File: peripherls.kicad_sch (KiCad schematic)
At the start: 14 parts, among them SW1 SW_MEC_5E, SW3 SW_MEC_5E, U2 STM32G070KBTx

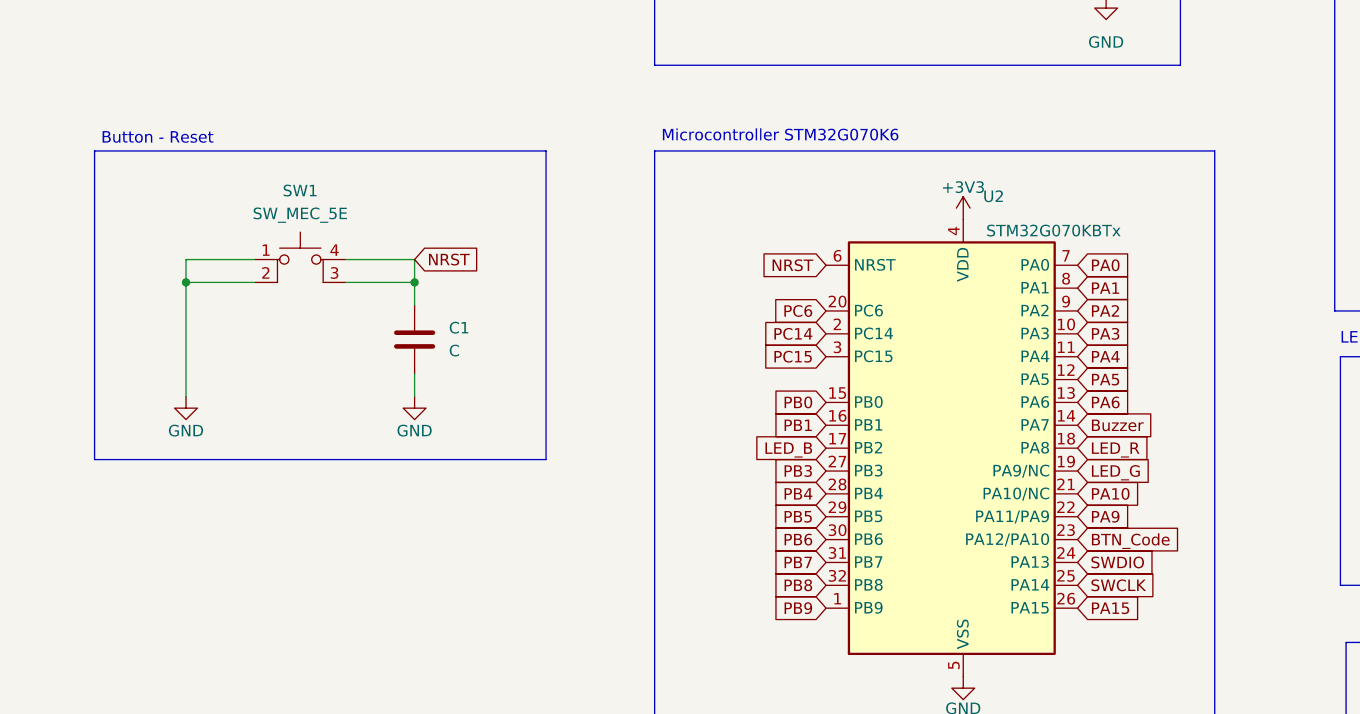
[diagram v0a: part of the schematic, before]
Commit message: [feat] PCB routing
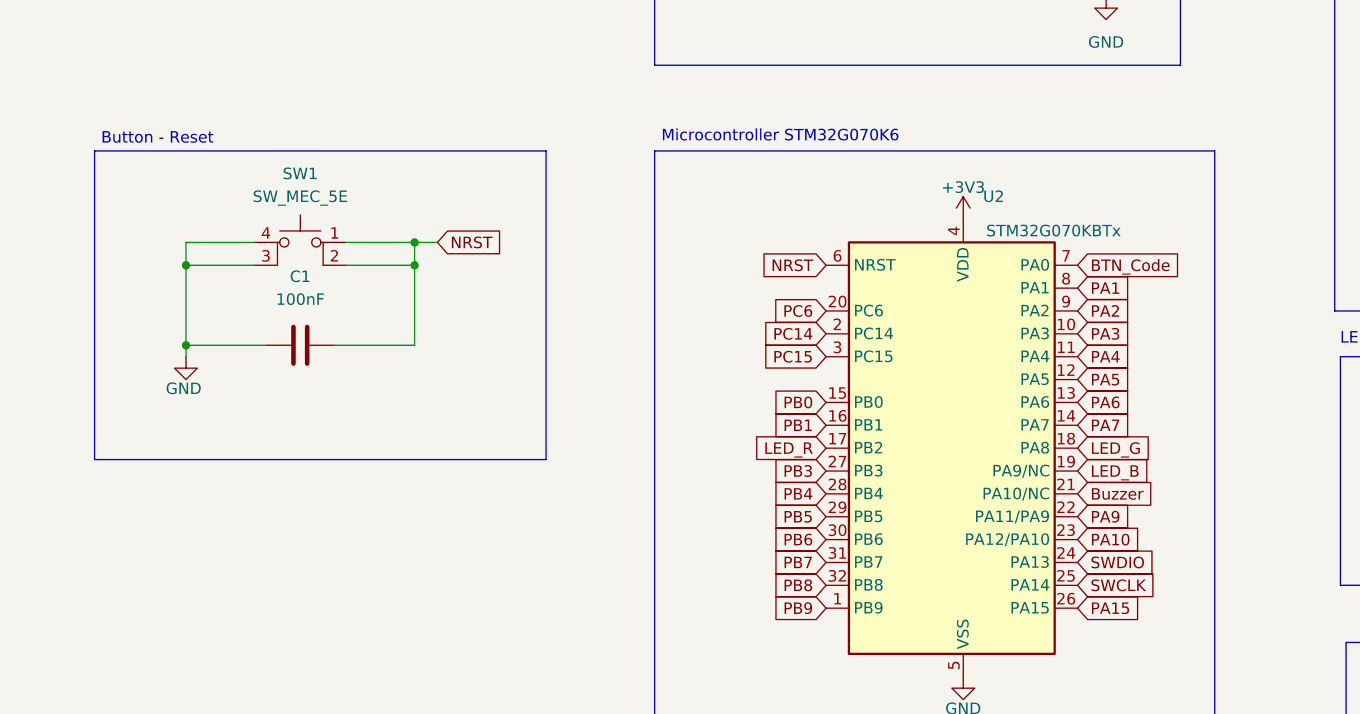
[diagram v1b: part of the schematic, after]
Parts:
- C1: value C -> 100nF
- D1: footprint LED_THT:LED_D1.8mm_W1.8mm_H2.4mm_Horizontal_O3.81mm_Z4.9mm -> LED_THT:LED_D2.0mm_W4.8mm_H2.5mm_FlatTop
- R2: footprint R_Axial_DIN0204_L3.6mm_D1.6mm_P7.62mm_Horizontal -> Resistor_THT:R_Axial_DIN0207_L6.3mm_D2.5mm_P7.62mm_Horizontal
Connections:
- net PA0 is gone; now on net BTN_Code: U2.7 (PA0)
- net BTN_Code: no longer U2.23 (PA12/PA10)
- net Buzzer: now also U2.21 (PA10/NC); no longer U2.14 (PA7)
- net GND: now also C1.1, SW1.3 (K), SW1.4 (A); no longer C1.2, SW1.1, SW1.2
- net LED_B: now also U2.19 (PA9/NC); no longer U2.17 (PB2)
- net LED_G: now also U2.18 (PA8); no longer U2.19 (PA9/NC)
- net LED_R: now also U2.17 (PB2); no longer U2.18 (PA8)
- net NRST: now also C1.2, SW1.1, SW1.2; no longer C1.1, SW1.3 (K), SW1.4 (A)
- net PA10: now also U2.23 (PA12/PA10); no longer U2.21 (PA10/NC)
- new net PA7: U2.14 (PA7)
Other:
- moved on the sheet: C1, SW1

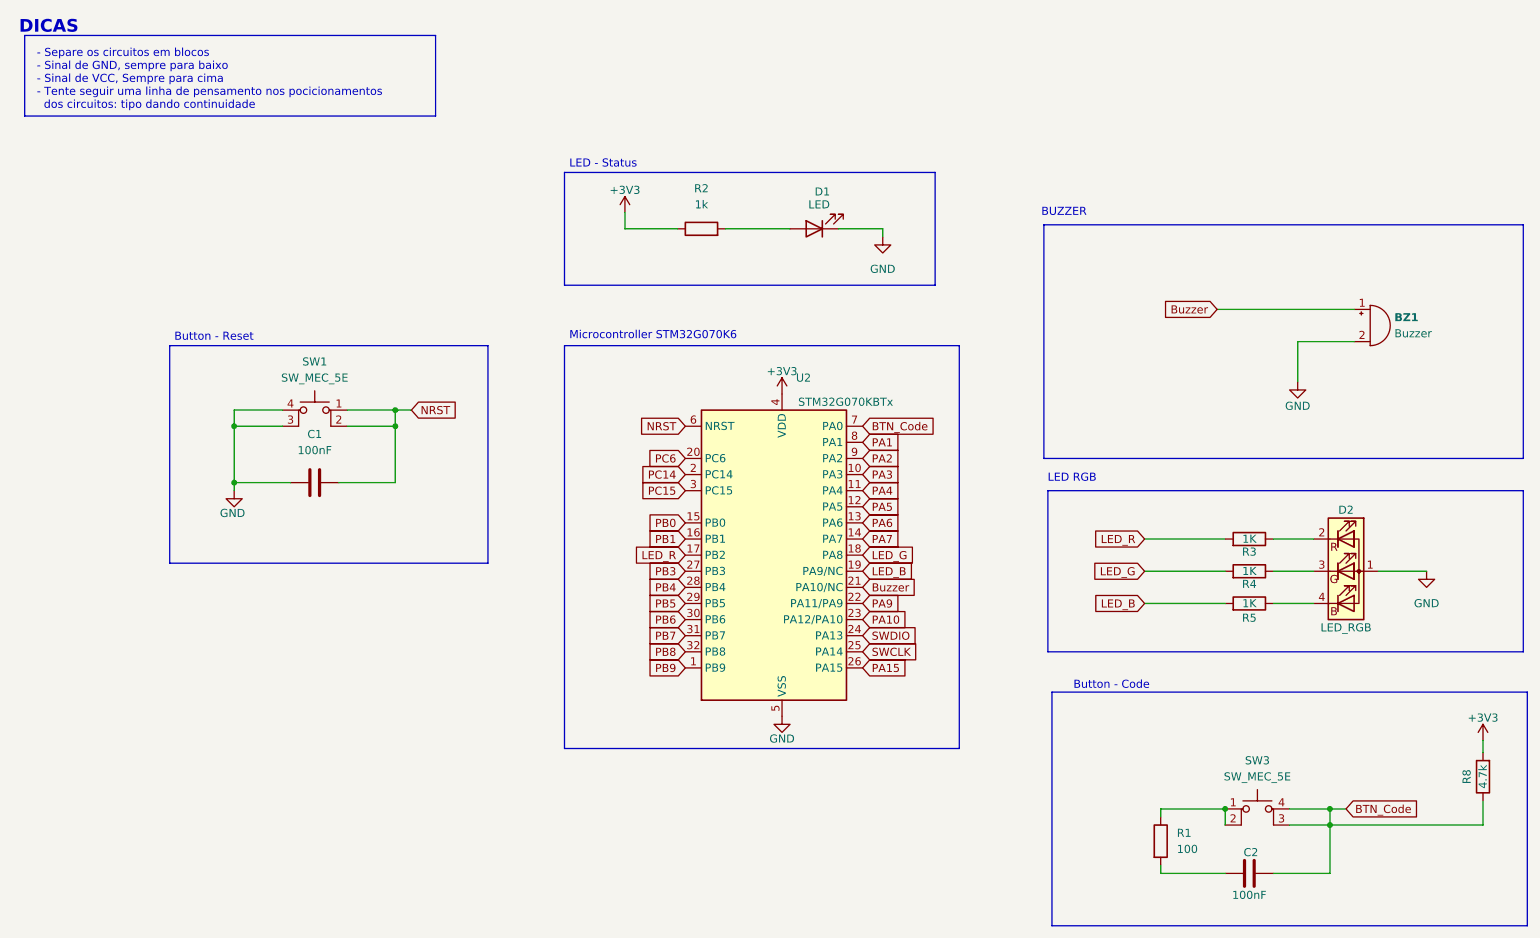
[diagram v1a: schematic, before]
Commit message: Modifying footprint positions
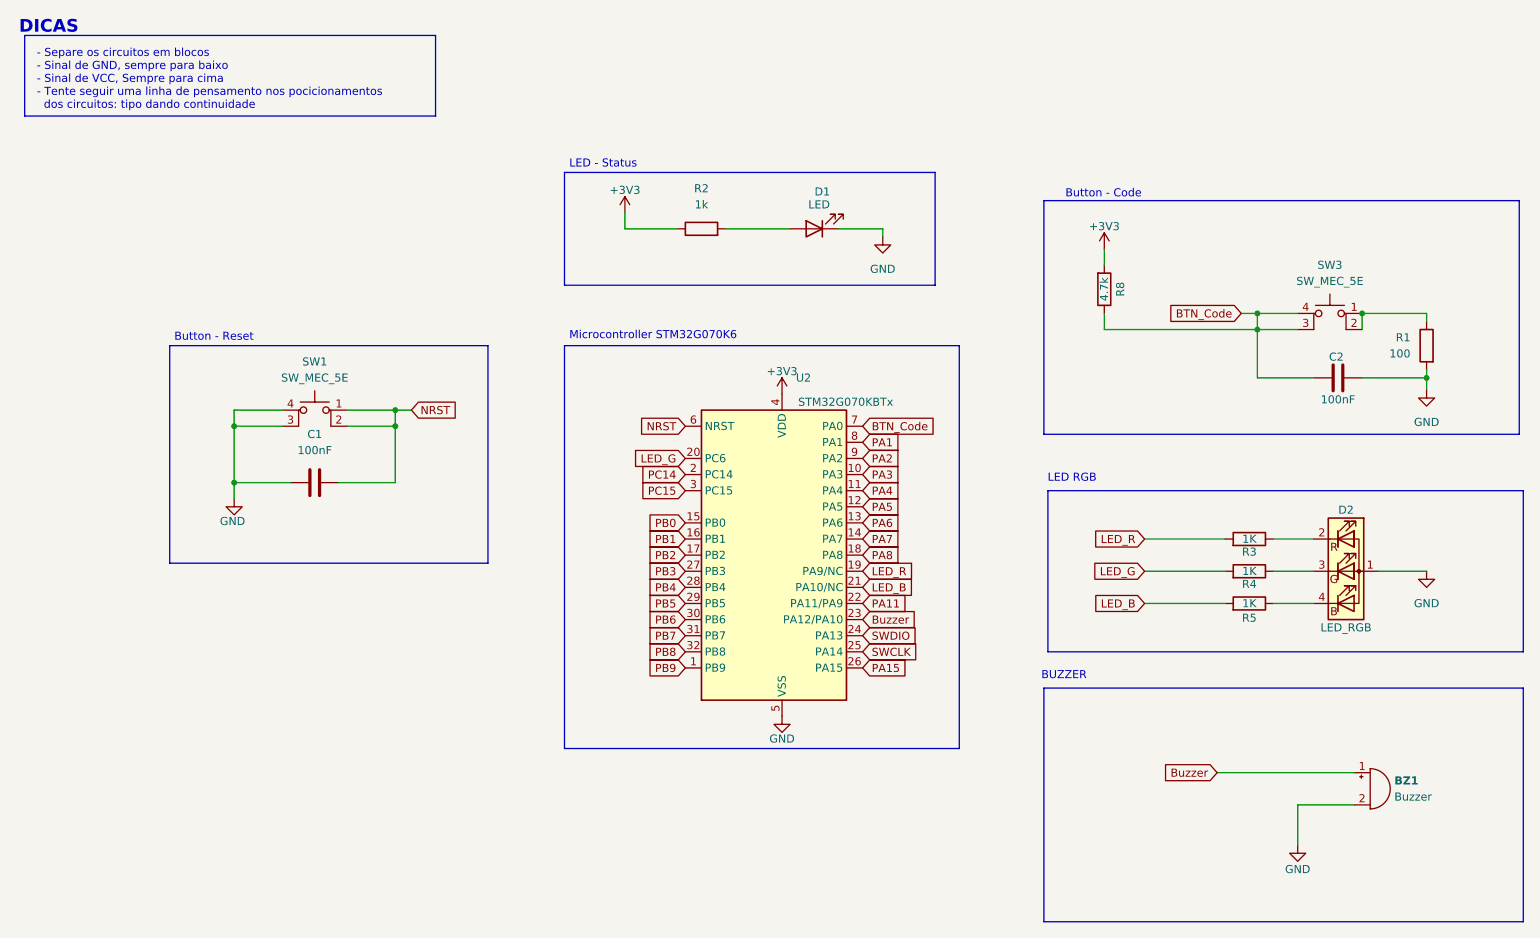
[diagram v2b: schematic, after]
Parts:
- SW1, SW3: footprint SW_PUSH-12mm_Wuerth-430476085716 -> personalized:SW_PUSH-12mm
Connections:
- net PA10 is gone; now on net Buzzer: U2.23 (PA12/PA10)
- net PC6 is gone; now on net LED_G: U2.20 (PC6)
- net Buzzer: no longer U2.21 (PA10/NC)
- net GND: now also C2.1, R1.2
- net LED_B: now also U2.21 (PA10/NC); no longer U2.19 (PA9/NC)
- net LED_G: no longer U2.18 (PA8)
- net LED_R: now also U2.19 (PA9/NC); no longer U2.17 (PB2)
- net PA9 renamed PA11
- new net PA8: U2.18 (PA8)
- new net PB2: U2.17 (PB2)
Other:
- moved on the sheet: BZ1, C2, R1, R8, SW3

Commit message: done - V1
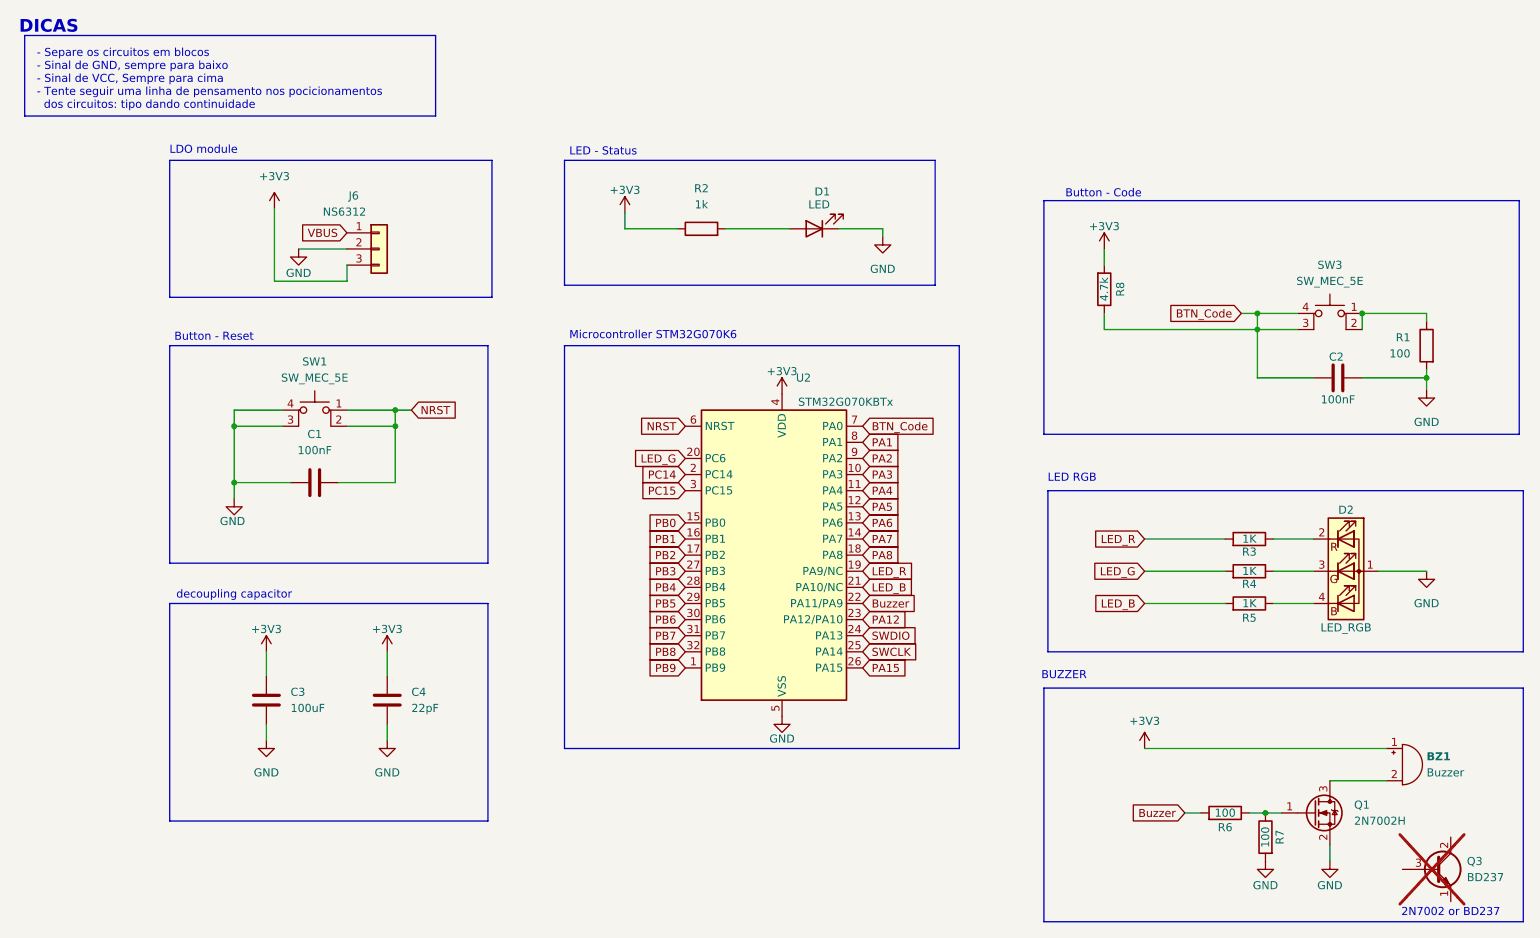
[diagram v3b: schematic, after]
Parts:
- added C3: 100uF, Capacitor_THT:CP_Radial_D8.0mm_P3.50mm, symbol Device:C
- added C4: 22pF, Capacitor_THT:CP_Radial_Tantal_D4.5mm_P5.00mm, symbol Device:C
- added J6: NS6312, Connector_PinHeader_2.54mm:PinHeader_1x03_P2.54mm_Vertical, symbol Connector_Generic:Conn_01x03
- added Q1: 2N7002H, Package_TO_SOT_THT:TO-251-3_Vertical, symbol Transistor_FET:2N7002H
- added Q3: BD237, Package_TO_SOT_THT:TO-18-3_Window, symbol Transistor_BJT:BD237
- added R6, R7: 100, Resistor_THT:R_Axial_DIN0207_L6.3mm_D2.5mm_P7.62mm_Horizontal, symbol Device:R
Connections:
- net PA11 is gone; now on net Buzzer: U2.22 (PA11/PA9)
- net +3V3: now also BZ1.1 (+), C3.1, C4.1, J6.3 (Pin_3)
- net Buzzer: now also R6.2; no longer BZ1.1 (+), U2.23 (PA12/PA10)
- net GND: now also C3.2, C4.2, J6.2 (Pin_2), Q1.2 (S), R7.2; no longer BZ1.2 (-)
- new net: Q1.1 (G), R6.1, R7.1
- new net: BZ1.2 (-), Q1.3 (D)
- new net PA12: U2.23 (PA12/PA10)
- new net VBUS: J6.1 (Pin_1)
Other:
- note added: "2N7002 or BD237"
- note added: "LDO module"
- note added: "decoupling capacitor"
- moved on the sheet: BZ1

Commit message: bugs
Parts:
- D2: footprint LED_THT:LED_D5.0mm-4_RGB_Wide_Pins -> personalized:LED_RGB
- R8: footprint (none) -> Resistor_THT:R_Axial_DIN0207_L6.3mm_D2.5mm_P7.62mm_Horizontal
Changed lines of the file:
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@@
 			)
 		)
-		(property "Footprint" "LED_THT:LED_D5.0mm-4_RGB_Wide_Pins"
+		(property "Footprint" "personalized:LED_RGB"
 			(at 223.52 102.87 0)
 			(effects
@@
 			)
 		)
-		(property "Footprint" ""
+		(property "Footprint" "Resistor_THT:R_Axial_DIN0207_L6.3mm_D2.5mm_P7.62mm_Horizontal"
 			(at 183.642 57.15 90)
 			(effects

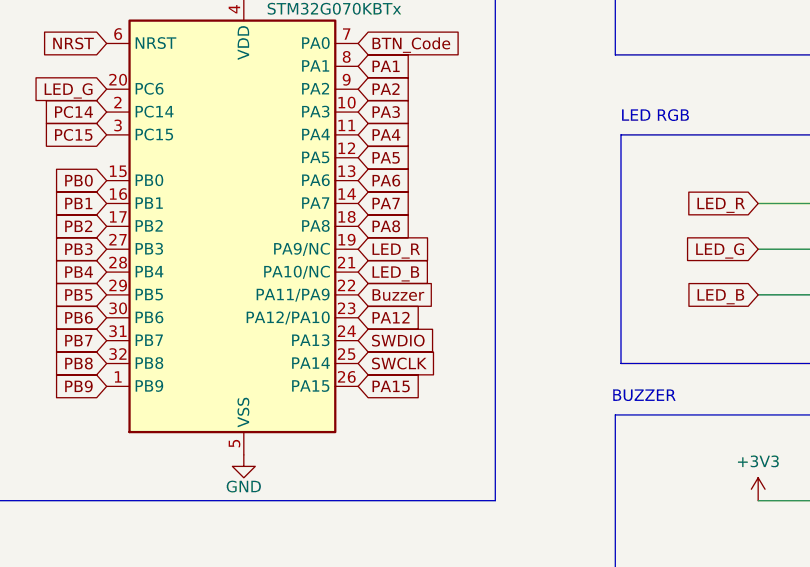
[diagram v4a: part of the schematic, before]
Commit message: perf: 45° micro
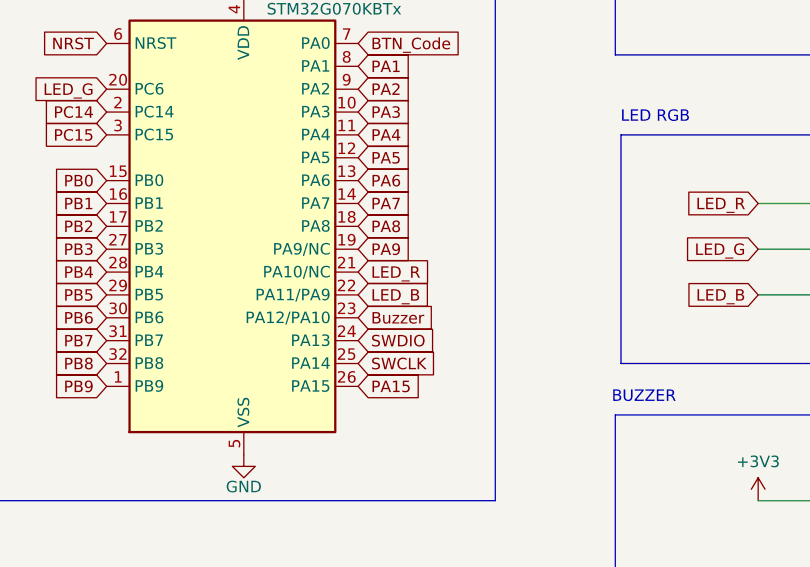
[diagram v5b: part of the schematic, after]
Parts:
- C1, C2: footprint C_Disc_D3.0mm_W1.6mm_P2.50mm -> personalized:C_Disc_D1mm
- C3: footprint Capacitor_THT:CP_Radial_D8.0mm_P3.50mm -> personalized:CP_Radial_1mm
- C4: footprint Capacitor_THT:CP_Radial_Tantal_D4.5mm_P5.00mm -> CP_Radial_Tantal_1mm
- D1: footprint LED_THT:LED_D2.0mm_W4.8mm_H2.5mm_FlatTop -> personalized:LED_1mm
- R1, R2, R3, R4, R5, R6, R7, R8: footprint Resistor_THT:R_Axial_DIN0207_L6.3mm_D2.5mm_P7.62mm_Horizontal -> Resistor_THT_Horizontal_1mm
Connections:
- net PA12 is gone; now on net Buzzer: U2.23 (PA12/PA10)
- net Buzzer: no longer U2.22 (PA11/PA9)
- net LED_B: now also U2.22 (PA11/PA9); no longer U2.21 (PA10/NC)
- net LED_R: now also U2.21 (PA10/NC); no longer U2.19 (PA9/NC)
- new net PA9: U2.19 (PA9/NC)
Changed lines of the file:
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@@
 	(global_label "Buzzer"
 		(shape input)
-		(at 147.32 106.68 0)
+		(at 147.32 109.22 0)
 		(fields_autoplaced yes)
 		(effects
@@
 		)
 		(property "Intersheetrefs" "${INTERSHEET_REFS}"
-			(at 156.6552 106.68 0)
+			(at 156.6552 109.22 0)
 			(effects
 				(font
@@
 		)
 	)
-	(global_label "PA12"
+	(global_label "PA9"
 		(shape input)
-		(at 147.32 109.22 0)
+		(at 147.32 101.6 0)
 		(fields_autoplaced yes)
 		(effects
@@
 		)
 		(property "Intersheetrefs" "${INTERSHEET_REFS}"
-			(at 155.0828 109.22 0)
+			(at 153.8733 101.6 0)
 			(effects
 				(font
@@
 	(global_label "LED_R"
 		(shape input)
-		(at 147.32 101.6 0)
+		(at 147.32 104.14 0)
 		(fields_autoplaced yes)
 		(effects
@@
 		)
 		(property "Intersheetrefs" "${INTERSHEET_REFS}"
-			(at 155.9899 101.6 0)
+			(at 155.9899 104.14 0)
 			(effects
 				(font
@@
 	(global_label "LED_B"
 		(shape input)
-		(at 147.32 104.14 0)
+		(at 147.32 106.68 0)
 		(fields_autoplaced yes)
 		(effects
@@
 		)
 		(property "Intersheetrefs" "${INTERSHEET_REFS}"
-			(at 155.9899 104.14 0)
+			(at 155.9899 106.68 0)
 			(effects
 				(font
@@
 			)
 		)
-		(property "Footprint" "Resistor_THT:R_Axial_DIN0207_L6.3mm_D2.5mm_P7.62mm_Horizontal"
+		(property "Footprint" "Resistor_THT_Horizontal_1mm"
 			(at 214.63 143.51 90)
 			(effects
@@
 			)
 		)
-		(property "Footprint" "C_Disc_D3.0mm_W1.6mm_P2.50mm"
+		(property "Footprint" "personalized:C_Disc_D1mm"
 			(at 218.44 70.1548 0)
 			(effects
@@
 			)
 		)
-		(property "Footprint" "Capacitor_THT:CP_Radial_Tantal_D4.5mm_P5.00mm"
+		(property "Footprint" "CP_Radial_Tantal_1mm"
 			(at 73.3552 125.73 0)
 			(effects
@@
 			)
 		)
-		(property "Footprint" "Resistor_THT:R_Axial_DIN0207_L6.3mm_D2.5mm_P7.62mm_Horizontal"
+		(property "Footprint" "Resistor_THT_Horizontal_1mm"
 			(at 208.28 104.14 90)
 			(effects
@@
 			)
 		)
-		(property "Footprint" "C_Disc_D3.0mm_W1.6mm_P2.50mm"
+		(property "Footprint" "personalized:C_Disc_D1mm"
 			(at 64.77 86.6648 0)
 			(effects
@@
 			)
 		)
-		(property "Footprint" "Resistor_THT:R_Axial_DIN0207_L6.3mm_D2.5mm_P7.62mm_Horizontal"
+		(property "Footprint" "Resistor_THT_Horizontal_1mm"
 			(at 208.28 110.49 90)
 			(effects
@@
 			)
 		)
-		(property "Footprint" "Resistor_THT:R_Axial_DIN0207_L6.3mm_D2.5mm_P7.62mm_Horizontal"
+		(property "Footprint" "Resistor_THT_Horizontal_1mm"
 			(at 121.92 49.403 90)
 			(effects
@@
 			)
 		)
-		(property "Footprint" "Resistor_THT:R_Axial_DIN0207_L6.3mm_D2.5mm_P7.62mm_Horizontal"
+		(property "Footprint" "Resistor_THT_Horizontal_1mm"
 			(at 204.47 143.51 90)
 			(effects
@@
 			)
 		)
-		(property "Footprint" "Resistor_THT:R_Axial_DIN0207_L6.3mm_D2.5mm_P7.62mm_Horizontal"
+		(property "Footprint" "Resistor_THT_Horizontal_1mm"
 			(at 183.642 57.15 90)
 			(effects
@@
 			)
 		)
-		(property "Footprint" "Capacitor_THT:CP_Radial_D8.0mm_P3.50mm"
+		(property "Footprint" "personalized:CP_Radial_1mm"
 			(at 54.3052 125.73 0)
 			(effects
@@
 			)
 		)
-		(property "Footprint" "Resistor_THT:R_Axial_DIN0207_L6.3mm_D2.5mm_P7.62mm_Horizontal"
+		(property "Footprint" "Resistor_THT_Horizontal_1mm"
 			(at 237.998 66.04 90)
 			(effects
@@
 			)
 		)
-		(property "Footprint" "Resistor_THT:R_Axial_DIN0207_L6.3mm_D2.5mm_P7.62mm_Horizontal"
+		(property "Footprint" "Resistor_THT_Horizontal_1mm"
 			(at 208.28 99.06 90)
 			(effects
@@
 			)
 		)
-		(property "Footprint" "LED_THT:LED_D2.0mm_W4.8mm_H2.5mm_FlatTop"
+		(property "Footprint" "personalized:LED_1mm"
 			(at 139.7 47.625 0)
 			(effects
